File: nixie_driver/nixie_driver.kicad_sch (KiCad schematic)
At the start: 23 parts, among them J1 USB_B_Micro, J10 Screw_Terminal_01x02, J11 Screw_Terminal_01x02, J12 Screw_Terminal_01x02, J2 GPIO, J3 HV_TEST, J4 Screw_Terminal_01x02, J5 Conn_01x11_Pin, J6 Conn_01x11_Pin, J7 Conn_01x11_Pin, J8 Conn_01x11_Pin, J9 Screw_Terminal_01x02, U1 SN74141N, U2 SN74141N, U3 SN74141N, U4 SN74141N

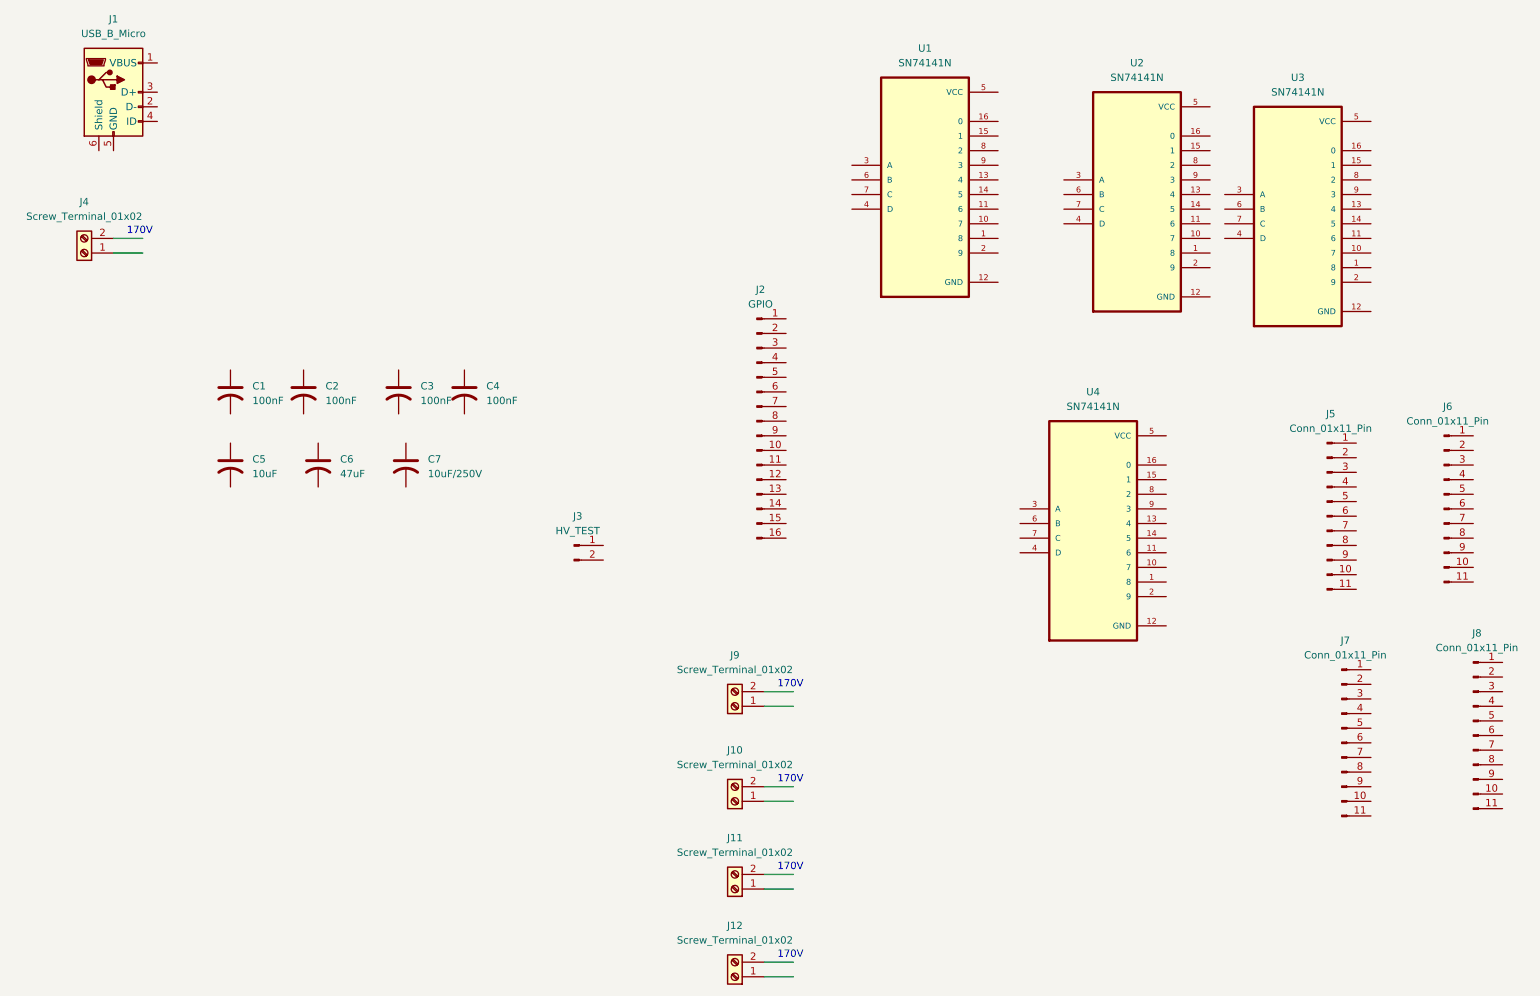
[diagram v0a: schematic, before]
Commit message: mostly done
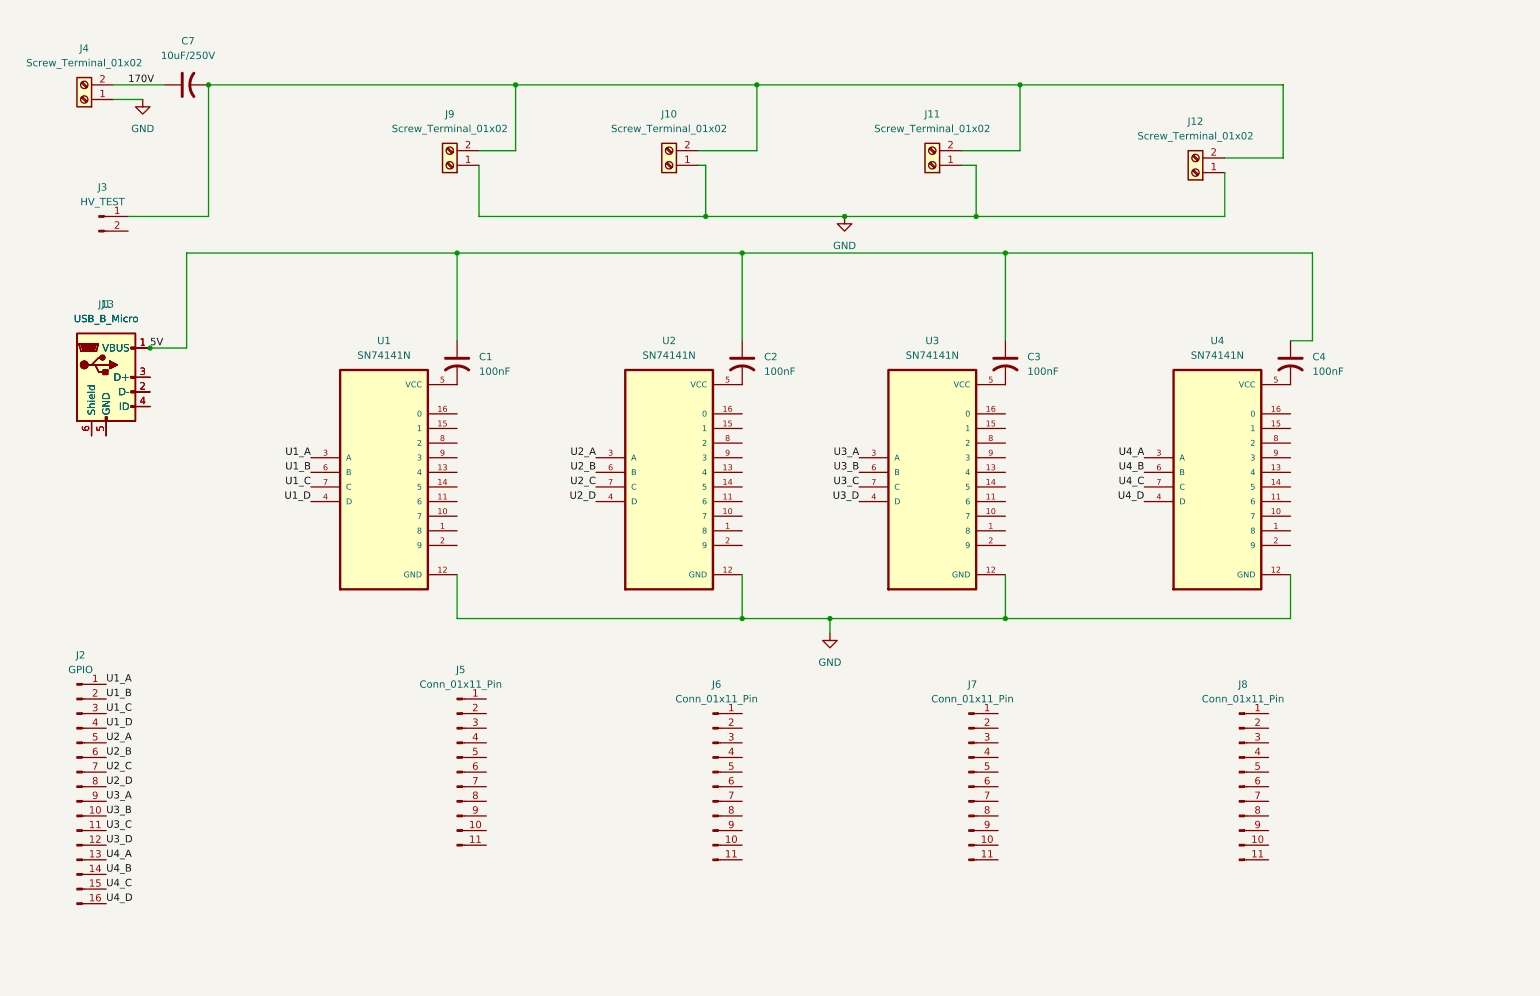
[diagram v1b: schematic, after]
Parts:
- removed C5: 10uF, symbol Device:C_US
- removed C6: 47uF, symbol Device:C_US
- added J13: USB_B_Micro, symbol Connector:USB_B_Micro
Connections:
- net GND: now reaches U1.12 (GND)
- net GND: now also J10.1 (Pin_1), J11.1 (Pin_1), J12.1 (Pin_1), J4.1 (Pin_1), J9.1 (Pin_1), U2.12 (GND), U3.12 (GND), U4.12 (GND)
- net U1_A: now reaches U1.3 (A)
- net U1_A: now also J2.1 (Pin_1)
- net U1_D: now reaches U1.4 (D)
- net U1_D: now also J2.4 (Pin_4)
- net at U1.5 (VCC): now also C1.2
- net U1_B: now reaches U1.6 (B)
- net U1_B: now also J2.2 (Pin_2)
- net U1_C: now reaches U1.7 (C)
- net U1_C: now also J2.3 (Pin_3)
- net 5V: now reaches C1.1
- net 5V: now also C2.1, C3.1, C4.1, J1.1 (VBUS), J13.1 (VBUS)
- net at J3.1 (Pin_1): now also C7.2, J10.2 (Pin_2), J11.2 (Pin_2), J12.2 (Pin_2), J9.2 (Pin_2)
- net at J1.2 (D-): now also J13.2 (D-)
- net at J1.3 (D+): now also J13.3 (D+)
- net at J1.4 (ID): now also J13.4 (ID)
- net at J1.5 (GND): now also J13.5 (GND)
- net at J1.6 (Shield): now also J13.6 (Shield)
- net 170V: now reaches C7.1
- net 170V: now also J4.2 (Pin_2)
- net U2_A: now reaches U2.3 (A)
- net U2_A: now also J2.5 (Pin_5)
- net U2_D: now reaches U2.4 (D)
- net U2_D: now also J2.8 (Pin_8)
- net at U2.5 (VCC): now also C2.2
- net U2_B: now reaches U2.6 (B)
- net U2_B: now also J2.6 (Pin_6)
- net U2_C: now reaches U2.7 (C)
- net U2_C: now also J2.7 (Pin_7)
- net at C3.2: now also U3.5 (VCC)
- net U3_B: now reaches J2.10 (Pin_10)
- net U3_B: now also U3.6 (B)
- net U3_C: now reaches J2.11 (Pin_11)
- net U3_C: now also U3.7 (C)
- net U3_D: now reaches J2.12 (Pin_12)
- net U3_D: now also U3.4 (D)
- net U4_A: now reaches J2.13 (Pin_13)
- net U4_A: now also U4.3 (A)
- net U4_B: now reaches J2.14 (Pin_14)
- net U4_B: now also U4.6 (B)
- net U4_C: now reaches J2.15 (Pin_15)
- net U4_C: now also U4.7 (C)
- net U4_D: now reaches J2.16 (Pin_16)
- net U4_D: now also U4.4 (D)
- net U3_A: now reaches J2.9 (Pin_9)
- net U3_A: now also U3.3 (A)
- net at U4.5 (VCC): now also C4.2
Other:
- note removed: "170V"
- moved on the sheet: C1, C2, C3, C4, C7, J10, J11, J12, J2, J3, J4, J5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
